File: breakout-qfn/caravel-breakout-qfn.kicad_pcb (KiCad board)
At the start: 2 copper layers, 45 x 52.5 mm, 79 parts, among them CON1 REF-182665-01, CON2 REF-182665-01, CON3 73251-1352, U1 Caravel_QFN

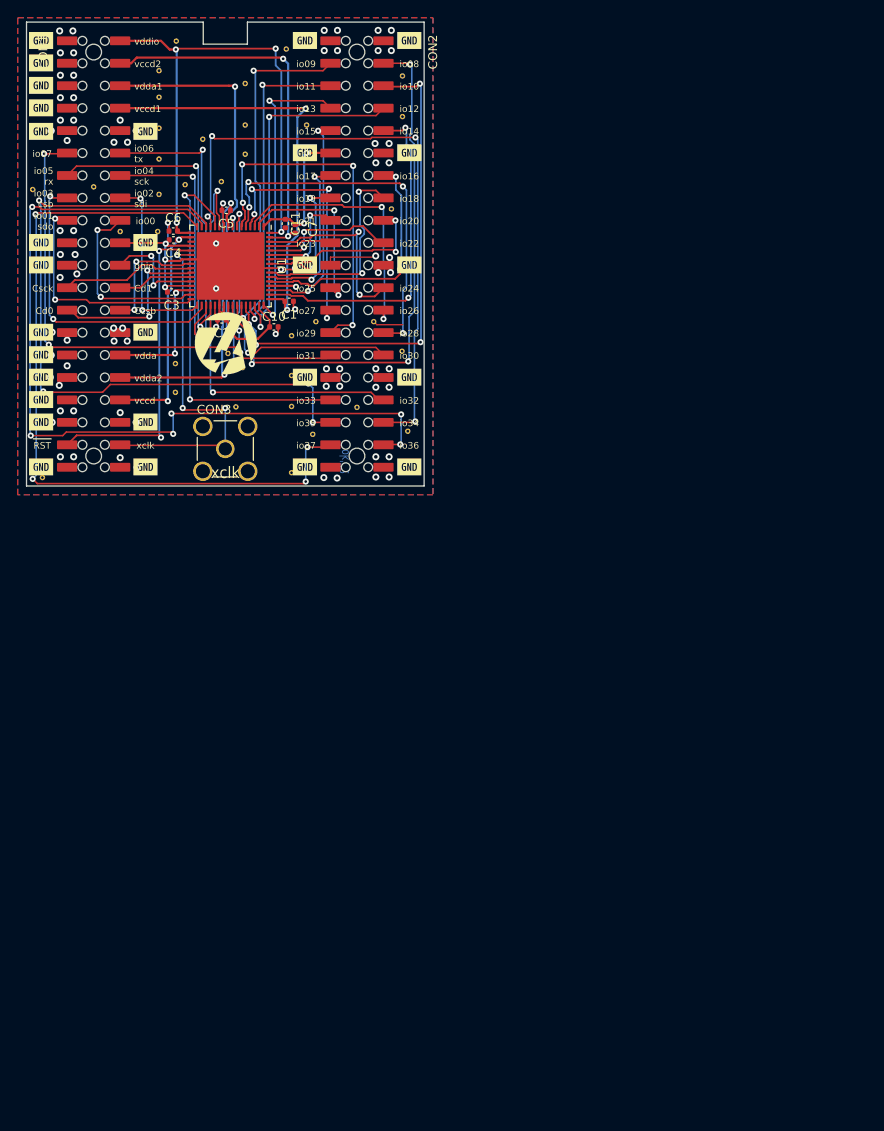
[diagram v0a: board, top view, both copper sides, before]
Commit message: sheet and origin cleanup
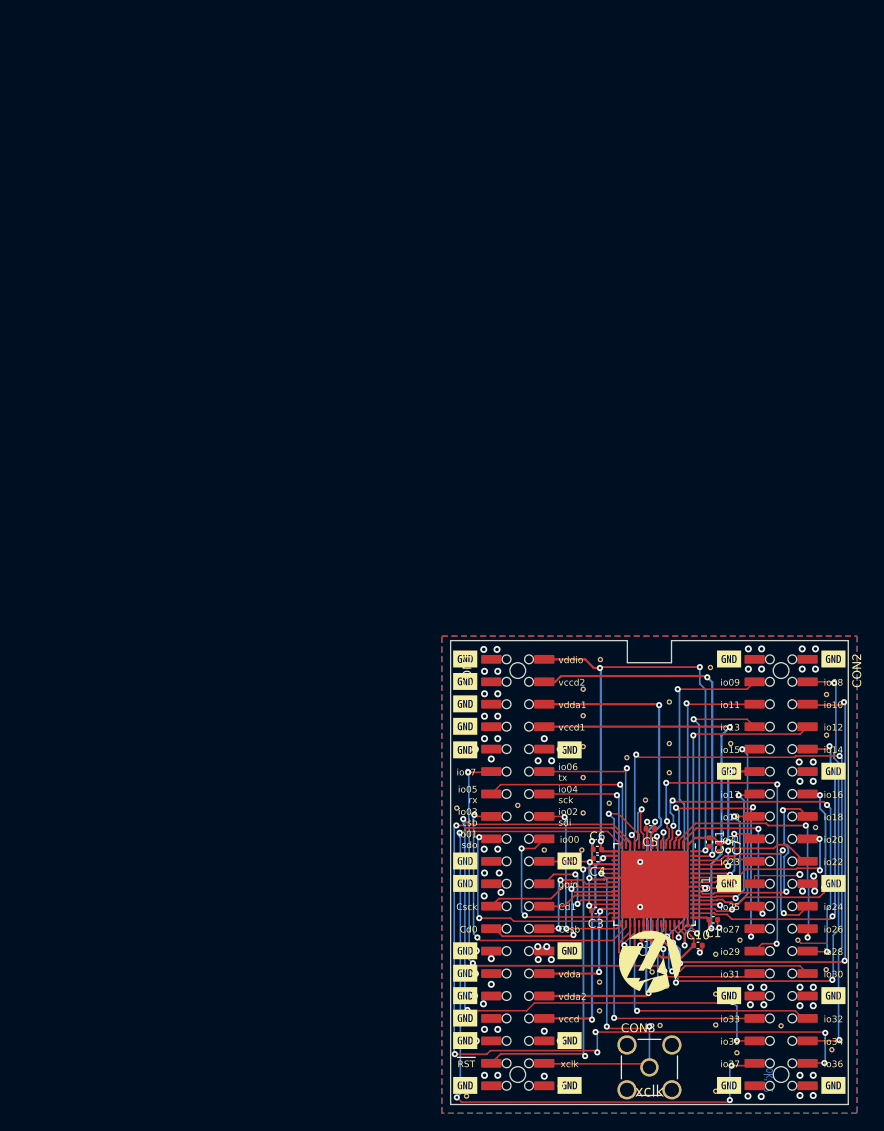
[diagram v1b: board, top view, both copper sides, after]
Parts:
- moved C1 84.9 mm to (77.7, 49.1)
- moved C10 84.9 mm to (76.0, 52.0)
- moved C11 84.9 mm to (77.3, 40.3)
- moved C2 84.9 mm to (70.1, 51.2)
- moved C3 84.9 mm to (64.4, 48.0)
- moved C4 84.9 mm to (64.6, 42.1)
- moved C5 84.9 mm to (70.6, 38.8)
- moved C6 84.9 mm to (64.6, 41.1)
- moved C7 84.9 mm to (78.4, 40.9)
- moved CON1 84.9 mm to (55.6, 43.8)
- moved CON2 84.9 mm to (85.4, 43.8)
- moved CON3 84.9 mm to (70.5, 65.8)
- moved REF** 84.9 mm to (90.5, 54.8)
- moved REF** 84.9 mm to (63.0, 37.0)
- moved REF** 84.9 mm to (63.0, 33.0)
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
